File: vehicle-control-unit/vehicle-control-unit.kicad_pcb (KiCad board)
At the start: 2 copper layers, 175.3 x 50.8 mm, 0 parts

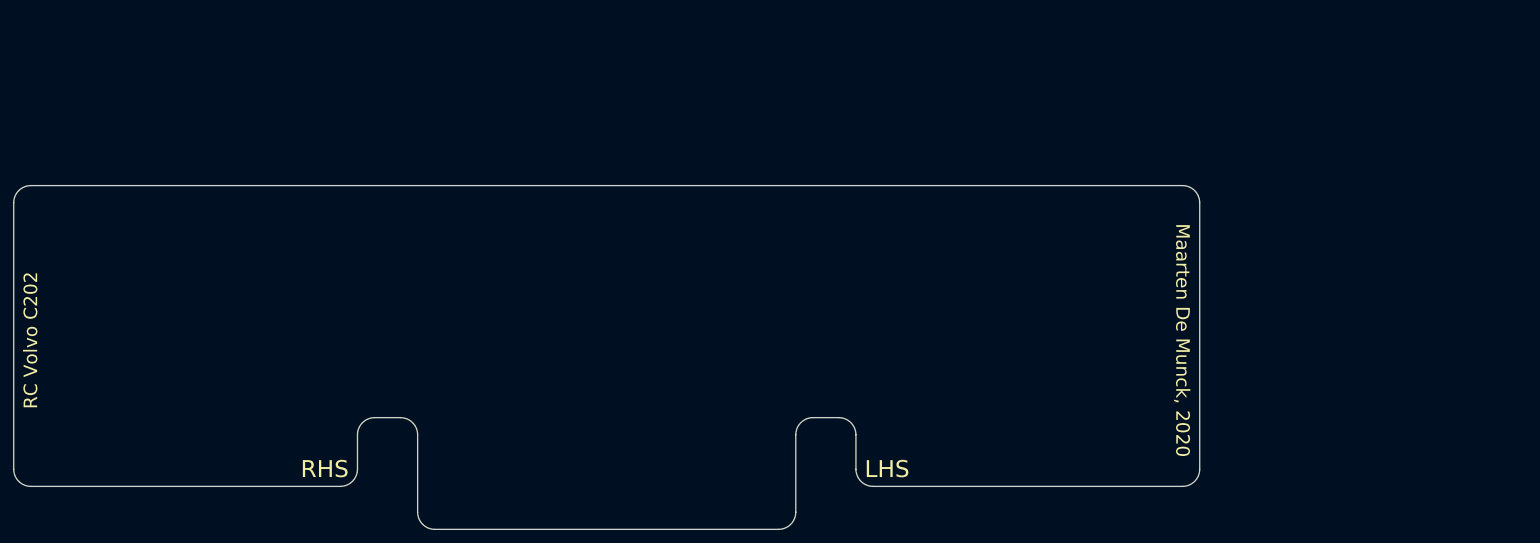
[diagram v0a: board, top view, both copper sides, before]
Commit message: Route PCB
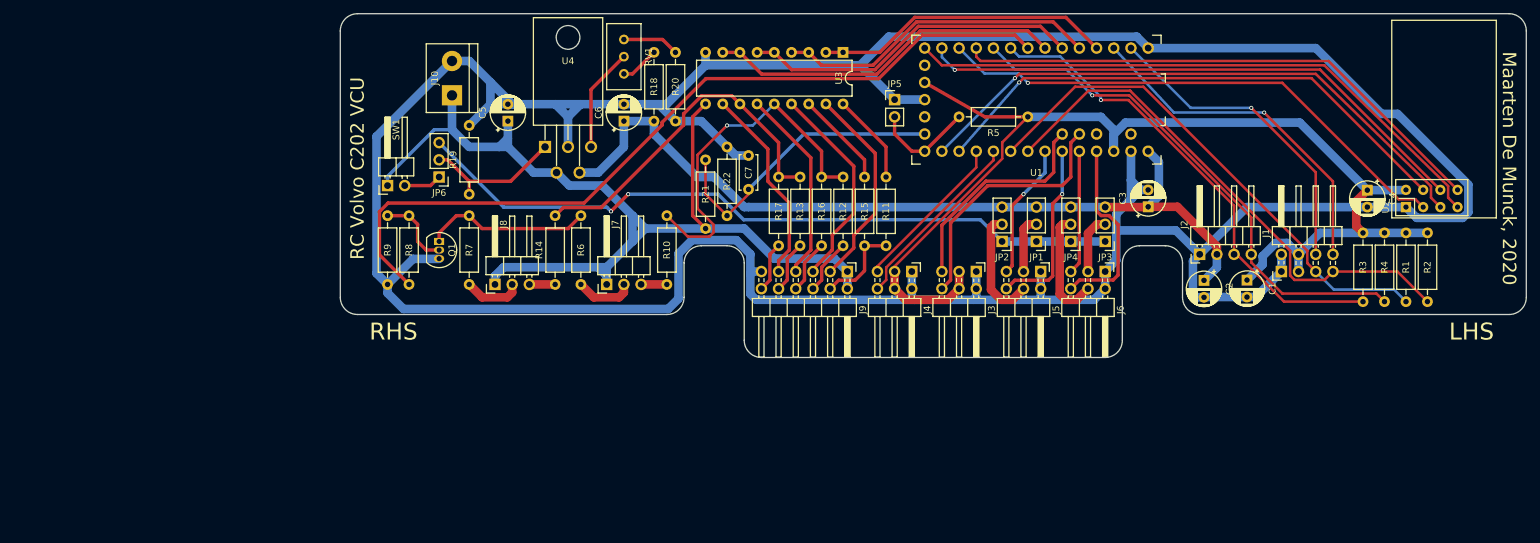
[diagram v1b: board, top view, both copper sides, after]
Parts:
- added C1: 10u, Capacitor_THT:CP_Radial_D5.0mm_P2.50mm, F.Cu at (200.0, 115.6)
- added C2: 10u, Capacitor_THT:CP_Radial_D5.0mm_P2.50mm, F.Cu at (193.7, 115.6)
- added C3: 10u, Capacitor_THT:CP_Radial_D5.0mm_P2.50mm, F.Cu at (185.4, 104.7)
- added C4: 10u, Capacitor_THT:CP_Radial_D5.0mm_P2.50mm, F.Cu at (217.8, 102.3)
- added C5: 10u, Capacitor_THT:CP_Radial_D5.0mm_P2.50mm, F.Cu at (90.8, 92.1)
- added C6: 22u, Capacitor_THT:CP_Radial_D5.0mm_P2.50mm, F.Cu at (108.0, 92.1)
- added C7: 100n, Capacitor_THT:C_Disc_D5.0mm_W2.5mm_P5.00mm, F.Cu at (126.4, 102.2)
- added J1: Conn_02x04_Male_UnitPerRow, Connector_PinHeader_2.54mm:PinHeader_2x04_P2.54mm_Horizontal, F.Cu at (205.1, 114.3)
- added J10: Connector:Screw_Terminal_01x02, TerminalBlock:TerminalBlock_bornier-2_P5.08mm, F.Cu at (82.5, 88.3)
- added J2: Conn_01x04_Male, Connector_PinHeader_2.54mm:PinHeader_1x04_P2.54mm_Horizontal, F.Cu at (193.0, 111.8)
- added J3: Conn_02x03_Male, Connector_PinHeader_2.54mm:PinHeader_2x03_P2.54mm_Horizontal, F.Cu at (160.0, 114.3)
- added J4: Conn_02x03_Male, Connector_PinHeader_2.54mm:PinHeader_2x03_P2.54mm_Horizontal, F.Cu at (150.5, 114.3)
- added J5: Conn_02x03_Male, Connector_PinHeader_2.54mm:PinHeader_2x03_P2.54mm_Horizontal, F.Cu at (169.5, 114.3)
- added J6: Conn_02x03_Male, Connector_PinHeader_2.54mm:PinHeader_2x03_P2.54mm_Horizontal, F.Cu at (179.1, 114.3)
- added J7: Conn_01x03_Male, Connector_PinHeader_2.54mm:PinHeader_1x03_P2.54mm_Horizontal, F.Cu at (105.4, 116.2)
- added J8: Conn_01x03_Male, Connector_PinHeader_2.54mm:PinHeader_1x03_P2.54mm_Horizontal, F.Cu at (88.9, 116.2)
- added J9: Conn_02x06_Male_UnitPerRow, Connector_PinHeader_2.54mm:PinHeader_2x06_P2.54mm_Horizontal, F.Cu at (141.0, 114.3)
- added JP1: Jumper_3_Bridged12, Connector_PinHeader_2.54mm:PinHeader_1x03_P2.54mm_Vertical, F.Cu at (168.9, 109.9)
- added JP2: Jumper_3_Bridged12, Connector_PinHeader_2.54mm:PinHeader_1x03_P2.54mm_Vertical, F.Cu at (163.8, 109.9)
- added JP3: Jumper_3_Bridged12, Connector_PinHeader_2.54mm:PinHeader_1x03_P2.54mm_Vertical, F.Cu at (179.1, 109.9)
- added JP4: Jumper_3_Bridged12, Connector_PinHeader_2.54mm:PinHeader_1x03_P2.54mm_Vertical, F.Cu at (174.0, 109.9)
- added JP5: Jumper_2_Open, Connector_PinHeader_2.54mm:PinHeader_1x02_P2.54mm_Vertical, F.Cu at (148.0, 88.9)
- added JP6: Jumper_3_Bridged12, Connector_PinHeader_2.54mm:PinHeader_1x03_P2.54mm_Vertical, F.Cu at (80.6, 100.3)
- added Q1: BC517, Package_TO_SOT_THT:TO-92_Inline, F.Cu at (80.6, 109.9)
- added R1: 10k, Resistor_THT:R_Axial_DIN0207_L6.3mm_D2.5mm_P10.16mm_Horizontal, F.Cu at (223.5, 108.6)
- added R10: 330E, Resistor_THT:R_Axial_DIN0207_L6.3mm_D2.5mm_P10.16mm_Horizontal, F.Cu at (114.3, 116.2)
- added R11: 470E, Resistor_THT:R_Axial_DIN0207_L6.3mm_D2.5mm_P10.16mm_Horizontal, F.Cu at (146.7, 110.5)
- added R12: 150E, Resistor_THT:R_Axial_DIN0207_L6.3mm_D2.5mm_P10.16mm_Horizontal, F.Cu at (140.3, 110.5)
- added R13: 150E, Resistor_THT:R_Axial_DIN0207_L6.3mm_D2.5mm_P10.16mm_Horizontal, F.Cu at (134.0, 110.5)
- added R14: 330E, Resistor_THT:R_Axial_DIN0207_L6.3mm_D2.5mm_P10.16mm_Horizontal, F.Cu at (97.8, 116.2)
- added R15: 82E, Resistor_THT:R_Axial_DIN0207_L6.3mm_D2.5mm_P10.16mm_Horizontal, F.Cu at (143.5, 110.5)
- added R16: 330E, Resistor_THT:R_Axial_DIN0207_L6.3mm_D2.5mm_P10.16mm_Horizontal, F.Cu at (137.2, 110.5)
- added R17: 330E, Resistor_THT:R_Axial_DIN0207_L6.3mm_D2.5mm_P10.16mm_Horizontal, F.Cu at (130.8, 110.5)
- added R18: 820E, Resistor_THT:R_Axial_DIN0207_L6.3mm_D2.5mm_P10.16mm_Horizontal, F.Cu at (112.4, 92.1)
- added R19: 10k, Resistor_THT:R_Axial_DIN0207_L6.3mm_D2.5mm_P10.16mm_Horizontal, F.Cu at (85.1, 102.9)
- added R2: 10k, Resistor_THT:R_Axial_DIN0207_L6.3mm_D2.5mm_P10.16mm_Horizontal, F.Cu at (226.7, 108.6)
- added R20: 240E, Resistor_THT:R_Axial_DIN0207_L6.3mm_D2.5mm_P10.16mm_Horizontal, F.Cu at (115.6, 81.9)
- added R21: 270k, 1%, Resistor_THT:R_Axial_DIN0207_L6.3mm_D2.5mm_P10.16mm_Horizontal, F.Cu at (120.0, 108.0)
- added R22: 100k, 1%, Resistor_THT:R_Axial_DIN0207_L6.3mm_D2.5mm_P10.16mm_Horizontal, F.Cu at (123.2, 106.0)
- added R3: 10k, Resistor_THT:R_Axial_DIN0207_L6.3mm_D2.5mm_P10.16mm_Horizontal, F.Cu at (217.2, 108.6)
- added R4: 10k, Resistor_THT:R_Axial_DIN0207_L6.3mm_D2.5mm_P10.16mm_Horizontal, F.Cu at (220.3, 108.6)
- added R5: 10k, Resistor_THT:R_Axial_DIN0207_L6.3mm_D2.5mm_P10.16mm_Horizontal, F.Cu at (167.6, 91.4)
- added R6: 10E, Resistor_THT:R_Axial_DIN0207_L6.3mm_D2.5mm_P10.16mm_Horizontal, F.Cu at (101.6, 116.2)
- added R7: 10E, Resistor_THT:R_Axial_DIN0207_L6.3mm_D2.5mm_P10.16mm_Horizontal, F.Cu at (85.1, 116.2)
- added R8: 10k, Resistor_THT:R_Axial_DIN0207_L6.3mm_D2.5mm_P10.16mm_Horizontal, F.Cu at (76.2, 106.0)
- added R9: 100k, Resistor_THT:R_Axial_DIN0207_L6.3mm_D2.5mm_P10.16mm_Horizontal, F.Cu at (73.0, 106.0)
- added RV1: 100E, Potentiometer_THT:Potentiometer_Bourns_3296W_Vertical, F.Cu at (108.0, 85.1)
- added SW1: SW_SPST, Connector_PinHeader_2.54mm:PinHeader_1x02_P2.54mm_Horizontal, F.Cu at (73.0, 101.6)
- added U1: Teensy3.2, earth-rover-footprints:Teensy_3.2, F.Cu at (168.9, 88.9)
- added U2: NRF24L01+ breakout, RF_Module:nRF24L01_Breakout, F.Cu at (223.5, 104.8)
- added U3: ULN2803A, Package_DIP:DIP-18_W7.62mm, F.Cu at (140.3, 81.9)
- added U4: MIC29502WT, Package_TO_SOT_THT:TO-220-5_P3.4x3.8mm_StaggerEven_Lead7.13mm_TabDown, F.Cu at (96.3, 95.9)
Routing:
- net GND: track 0.00 -> 515.8 mm
- net +3V3: track 0.00 -> 172.4 mm
- net +BATT: track 0.00 -> 148.6 mm
- net +5V: track 0.00 -> 123.7 mm
- net /HEADLAMPS: track 0.00 -> 120.2 mm
- net /BEC: track 0.00 -> 106.6 mm, vias 0 -> 2
- net /NRF24L01_MISO: track 0.00 -> 89.3 mm
- net /NRF24L01_SCK: track 0.00 -> 87.4 mm, vias 0 -> 1
- net /NRF24L01_MOSI: track 0.00 -> 83.2 mm, vias 0 -> 1
- net /NRF24L01_IRQ: track 0.00 -> 80.5 mm
- net /NRF24L01_CSN: track 0.00 -> 80.3 mm, vias 0 -> 1
- net /IMU_I2C_SCL: track 0.00 -> 78.8 mm
- net /NRF24L01_CE: track 0.00 -> 78.3 mm, vias 0 -> 1
- net /ENCODER_B: track 0.00 -> 77.2 mm, vias 0 -> 1
- net /IMU_I2C_SDA: track 0.00 -> 76.6 mm
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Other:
- outline, holes or cut-outs redrawn
- net class Default: trace_width 0.25 -> 0.2; via_dia 0.8 -> 0.6; via_drill 0.4 -> 0.35
- rule trace_min: 0.2 -> 0.15
- rule via_min_drill: 0.3 -> 0.35
- rule via_min_size: 0.4 -> 0.6
- board text added: "RC Volvo C202 VCU"
- board text removed: "RC Volvo C202"
